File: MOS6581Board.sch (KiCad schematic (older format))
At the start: 20 parts, among them J1 Board connector, J2 Power connector, U1 MOS6581, U2 LM7805_TO220, U3 MAX7375

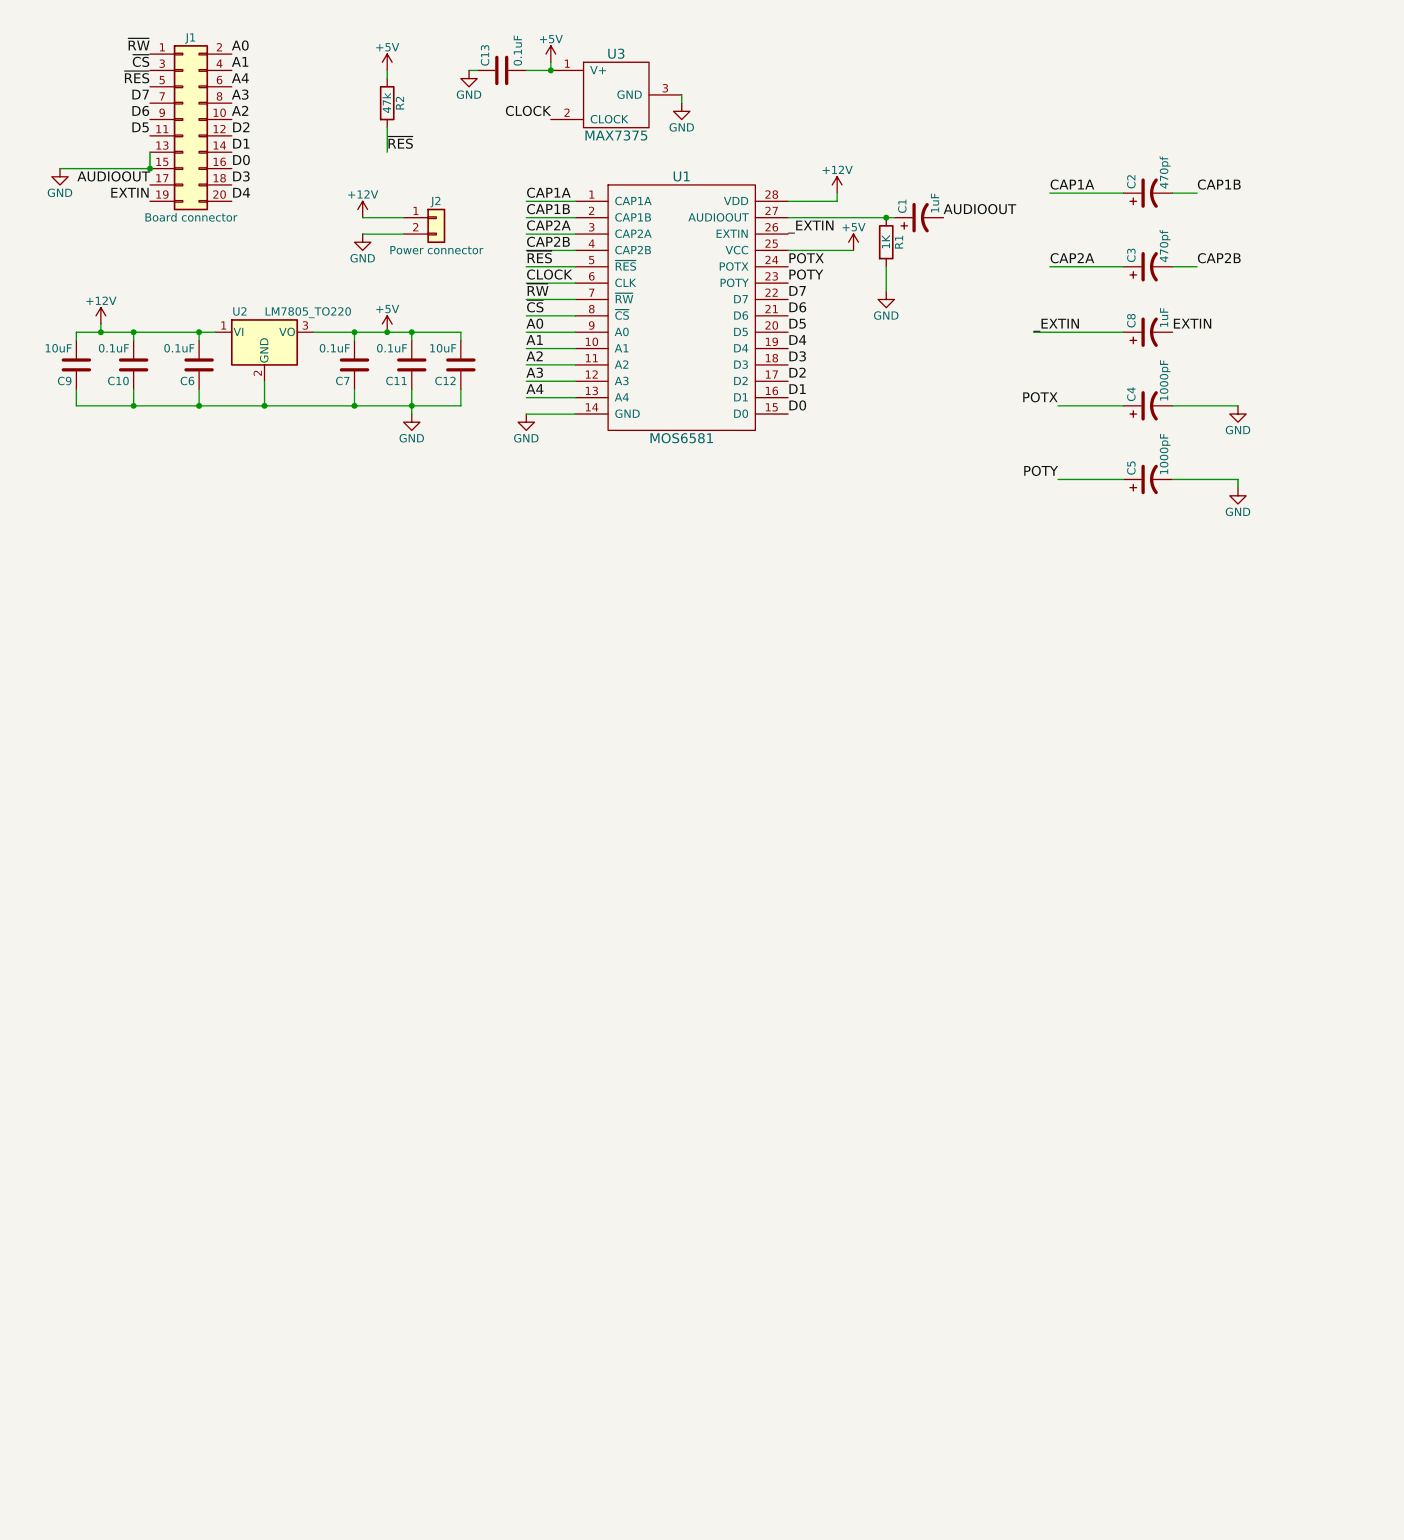
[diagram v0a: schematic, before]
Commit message: Add latest changes
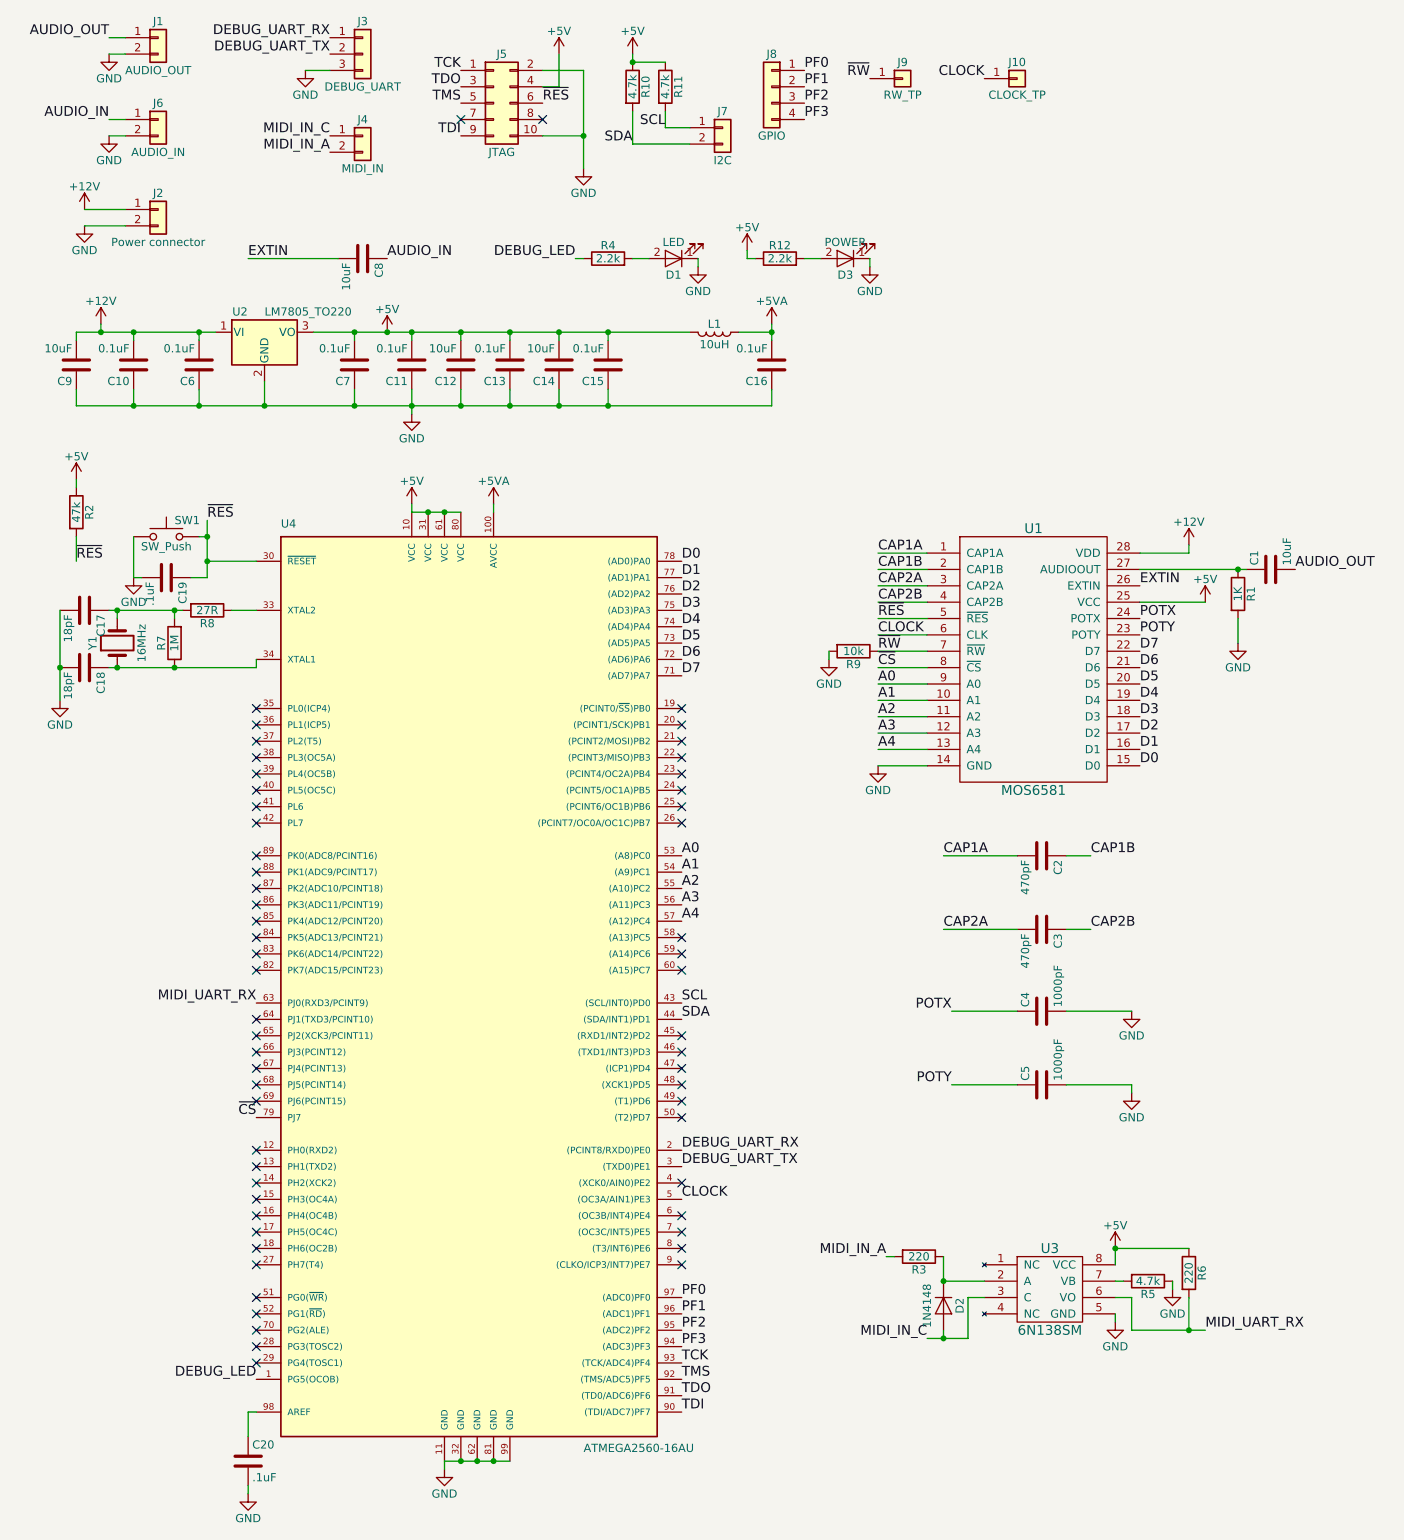
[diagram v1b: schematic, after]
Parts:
- removed C1, C8: 1uF, Capacitors_SMD:C_0805_HandSoldering, symbol CP1
- removed C2, C3: 470pf, Capacitors_SMD:C_0805_HandSoldering, symbol CP1
- removed C4, C5: 1000pF, Capacitors_SMD:C_0805_HandSoldering, symbol CP1
- removed J1: Board connector, Pin_Headers:Pin_Header_Straight_2x10_Pitch2.54mm, symbol Conn_02x10_Odd_Even
- removed U3: MAX7375, TO_SOT_Packages_SMD:SOT-323_SC-70_Handsoldering, symbol MAX7375
- added C1, C8: 10uF, Capacitors_THT:CP_Radial_D5.0mm_P2.50mm, symbol C
- added C14: 10uF, Capacitors_SMD:C_0805_HandSoldering, symbol C
- added C15, C16: 0.1uF, Capacitors_SMD:C_0805_HandSoldering, symbol C
- added C17, C18: 18pF, Capacitors_SMD:C_0805_HandSoldering, symbol C
- added C19, C20: .1uF, Capacitors_SMD:C_0805_HandSoldering, symbol C
- added C2, C3: 470pF, Resistors_THT:R_Axial_DIN0614_L14.3mm_D5.7mm_P20.32mm_Horizontal, symbol C
- added C4, C5: 1000pF, Capacitors_SMD:C_0805_HandSoldering, symbol C
- added D1: LED, LEDs:LED_0805_HandSoldering, symbol LED
- added D2: 1N4148, Diodes_SMD:D_SOD-323_HandSoldering, symbol D
- added D3: POWER, LEDs:LED_0805_HandSoldering, symbol LED
- added J1: AUDIO_OUT, Pin_Headers:Pin_Header_Straight_1x02_Pitch2.54mm, symbol Conn_01x02
- added J10: CLOCK_TP, Pin_Headers:Pin_Header_Straight_1x01_Pitch1.27mm, symbol Conn_01x01
- added J3: DEBUG_UART, Pin_Headers:Pin_Header_Straight_1x03_Pitch2.54mm, symbol Conn_01x03
- added J4: MIDI_IN, Pin_Headers:Pin_Header_Straight_1x02_Pitch2.54mm, symbol Conn_01x02
- added J5: JTAG, Pin_Headers:Pin_Header_Straight_2x05_Pitch2.54mm, symbol Conn_02x05_Odd_Even
- added J6: AUDIO_IN, Pin_Headers:Pin_Header_Straight_1x02_Pitch2.54mm, symbol Conn_01x02
- added J7: I2C, Pin_Headers:Pin_Header_Straight_1x02_Pitch2.54mm, symbol Conn_01x02
- added J8: GPIO, Pin_Headers:Pin_Header_Straight_1x04_Pitch1.27mm, symbol Conn_01x04
- added J9: RW_TP, Pin_Headers:Pin_Header_Straight_1x01_Pitch1.27mm, symbol Conn_01x01
- added L1: 10uH, Resistors_SMD:R_1206_HandSoldering, symbol L
- added R10, R11, R5: 4.7k, Resistors_SMD:R_0805_HandSoldering, symbol R
- added R12, R4: 2.2k, Resistors_SMD:R_0805_HandSoldering, symbol R
- added R3, R6: 220, Resistors_SMD:R_0805_HandSoldering, symbol R
- added R7: 1M, Resistors_SMD:R_0805_HandSoldering, symbol R
- added R8: 27R, Resistors_SMD:R_0805_HandSoldering, symbol R
- added R9: 10k, Resistors_SMD:R_0805_HandSoldering, symbol R
- added SW1: SW_Push, Buttons_Switches_THT:SW_PUSH_6mm, symbol SW_Push
- added U3: 6N138SM, Housings_DIP:SMDIP-8_W7.62mm, symbol 6N138SM
- added U4: ATMEGA2560-16AU, Housings_QFP:TQFP-100_14x14mm_Pitch0.5mm, symbol ATMEGA2560-16AU
- added Y1: 16MHz, Crystals:Crystal_SMD_HC49-SD_HandSoldering, symbol Crystal
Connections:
- net _EXTIN is gone; now on net EXTIN: U1.26 (EXTIN)
- net +5V: now also C14.2, C15.2, J5.4 (Pin_4), L1.2, R10.1, R11.1, R12.1, R6.1, U3.8 (VCC), U4.10 (VCC), U4.31 (VCC), U4.61 (VCC), U4.80 (VCC)
- net A0: now also U4.53 ((A8)PC0)
- net A1: now also U4.54 ((A9)PC1)
- net A2: now also U4.55 ((A10)PC2)
- net A3: now also U4.56 ((A11)PC3)
- net A4: now also U4.57 ((A12)PC4)
- net CAP1A: now also C2.2
- net CAP1B: now also C2.1
- net CAP2A: now also C3.2
- net CAP2B: now also C3.1
- net CLOCK: now also J10.1 (Pin_1), U4.5 ((OC3A/AIN1)PE3)
- net D0: now also U4.78 ((AD0)PA0)
- net D1: now also U4.77 ((AD1)PA1)
- net D2: now also U4.76 ((AD2)PA2)
- net D3: now also U4.75 ((AD3)PA3)
- net D4: now also U4.74 ((AD4)PA4)
- net D5: now also U4.73 ((AD5)PA5)
- net D6: now also U4.72 ((AD6)PA6)
- net D7: now also U4.71 ((AD7)PA7)
- net EXTIN: now also C8.2
- net GND: now also C14.1, C15.1, C16.1, C17.2, C18.2, C19.2, C20.2, C4.2, C5.2, D1.1 (K), D3.1 (K), J1.2 (Pin_2), J3.3 (Pin_3), J5.10 (Pin_10), J5.2 (Pin_2), J6.2 (Pin_2), R5.1, R9.2, SW1.1, U3.5 (GND), U4.11 (GND), U4.32 (GND), U4.62 (GND), U4.81 (GND), U4.99 (GND)
- net POTX: now also C4.1
- net POTY: now also C5.1
- net ~CS: now also U4.79 (PJ7)
- net ~RES: now also C19.1, J5.6 (Pin_6), SW1.2, U4.30 (~RESET)
- net ~RW: now also J9.1 (Pin_1), R9.1
- net at R1.1, U1.27 (AUDIOOUT): now also C1.1
- new net: R8.1, U4.33 (XTAL2)
- new net: C18.1, R7.1, U4.34 (XTAL1), Y1.1
- new net: C20.1, U4.98 (AREF)
- new net: C17.1, R7.2, R8.2, Y1.2
- new net: D1.2 (A), R4.2
- new net: D2.1 (K), R3.1, U3.2 (A)
- new net: R5.2, U3.7 (VB)
- new net: D3.2 (A), R12.2
- new net +5VA: C16.2, L1.1, U4.100 (AVCC)
- new net AUDIO_IN: C8.1, J6.1 (Pin_1)
- new net AUDIO_OUT: C1.2, J1.1 (Pin_1)
- new net DEBUG_LED: R4.1, U4.1 (PG5(OCOB))
- new net DEBUG_UART_RX: J3.1 (Pin_1), U4.2 ((PCINT8/RXD0)PE0)
- new net DEBUG_UART_TX: J3.2 (Pin_2), U4.3 ((TXD0)PE1)
- new net MIDI_IN_A: J4.2 (Pin_2), R3.2
- new net MIDI_IN_C: D2.2 (A), J4.1 (Pin_1), U3.3 (C)
- new net MIDI_UART_RX: R6.2, U3.6 (VO), U4.63 (PJ0(RXD3/PCINT9))
- new net PF0: J8.1 (Pin_1), U4.97 ((ADC0)PF0)
- new net PF1: J8.2 (Pin_2), U4.96 ((ADC1)PF1)
- new net PF2: J8.3 (Pin_3), U4.95 ((ADC2)PF2)
- new net PF3: J8.4 (Pin_4), U4.94 ((ADC3)PF3)
- new net SCL: J7.1 (Pin_1), R11.2, U4.43 ((SCL/INT0)PD0)
- new net SDA: J7.2 (Pin_2), R10.2, U4.44 ((SDA/INT1)PD1)
- new net TCK: J5.1 (Pin_1), U4.93 ((TCK/ADC4)PF4)
- new net TDI: J5.9 (Pin_9), U4.90 ((TDI/ADC7)PF7)
- new net TDO: J5.3 (Pin_3), U4.91 ((TD0/ADC6)PF6)
- new net TMS: J5.5 (Pin_5), U4.92 ((TMS/ADC5)PF5)
- no-connect marks 0 -> 59
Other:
- moved on the sheet: J2, R1, R2, U1
